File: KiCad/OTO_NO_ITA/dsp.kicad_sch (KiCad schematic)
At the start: 43 parts, among them J5 Conn_02x07_Odd_Even, J6 15910060, Q1 STD2805T4, SW4 SKRPABE010, U3 ADAU1466WBCPZ300RL, U4 ADM811TARTZ, X2 12.288MHz

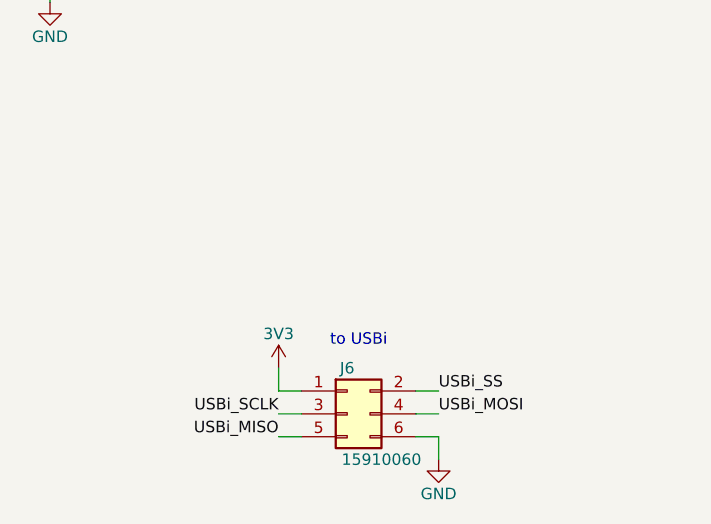
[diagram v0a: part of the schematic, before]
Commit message: Modified the pin header J6 for USBi.
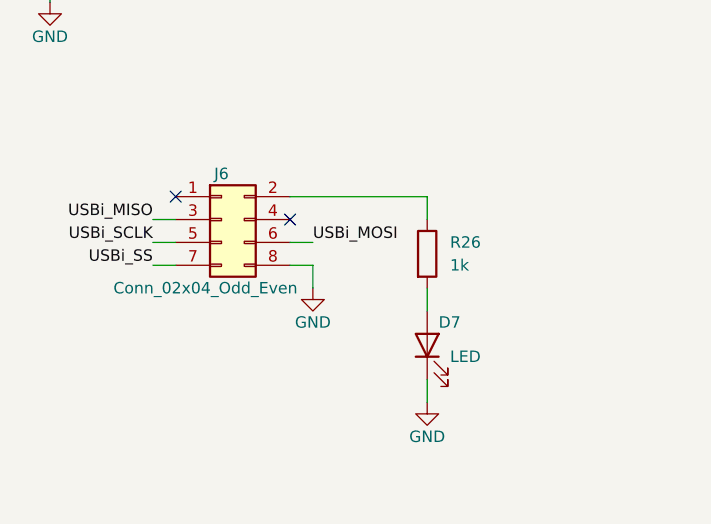
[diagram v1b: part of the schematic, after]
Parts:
- removed J6: 15910060, Connector_PinHeader_2.54mm:PinHeader_2x03_P2.54mm_Vertical, symbol Connector_Generic:Conn_02x03_Odd_Even
- added D7: LED, LED_SMD:LED_0603_1608Metric, symbol Device:LED
- added J6: Conn_02x04_Odd_Even, Connector_PinHeader_2.54mm:PinHeader_2x04_P2.54mm_Vertical, symbol Connector_Generic:Conn_02x04_Odd_Even
- added R26: 1k, Resistor_SMD:R_0201_0603Metric, symbol Device:R
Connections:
- net DSP_MISO: now also J6.3 (Pin_3)
- net DSP_MOSI: now also J6.6 (Pin_6)
- net DSP_SCLK: now also J6.5 (Pin_5)
- net DSP_SS: now also J6.7 (Pin_7)
- net GND: now also D7.1 (K), J6.8 (Pin_8)
- new net: J6.2 (Pin_2), R26.1
- new net: D7.2 (A), R26.2
- no-connect marks 28 -> 30
